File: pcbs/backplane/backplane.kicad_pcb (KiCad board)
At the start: 2 copper layers, 80 x 50 mm, 11 parts, among them P1 CONN_02X04, P2 CONN_02X04, P3 USB_B, P4 CONN_02X09, P5 CONN_02X09, U1 FT232RL

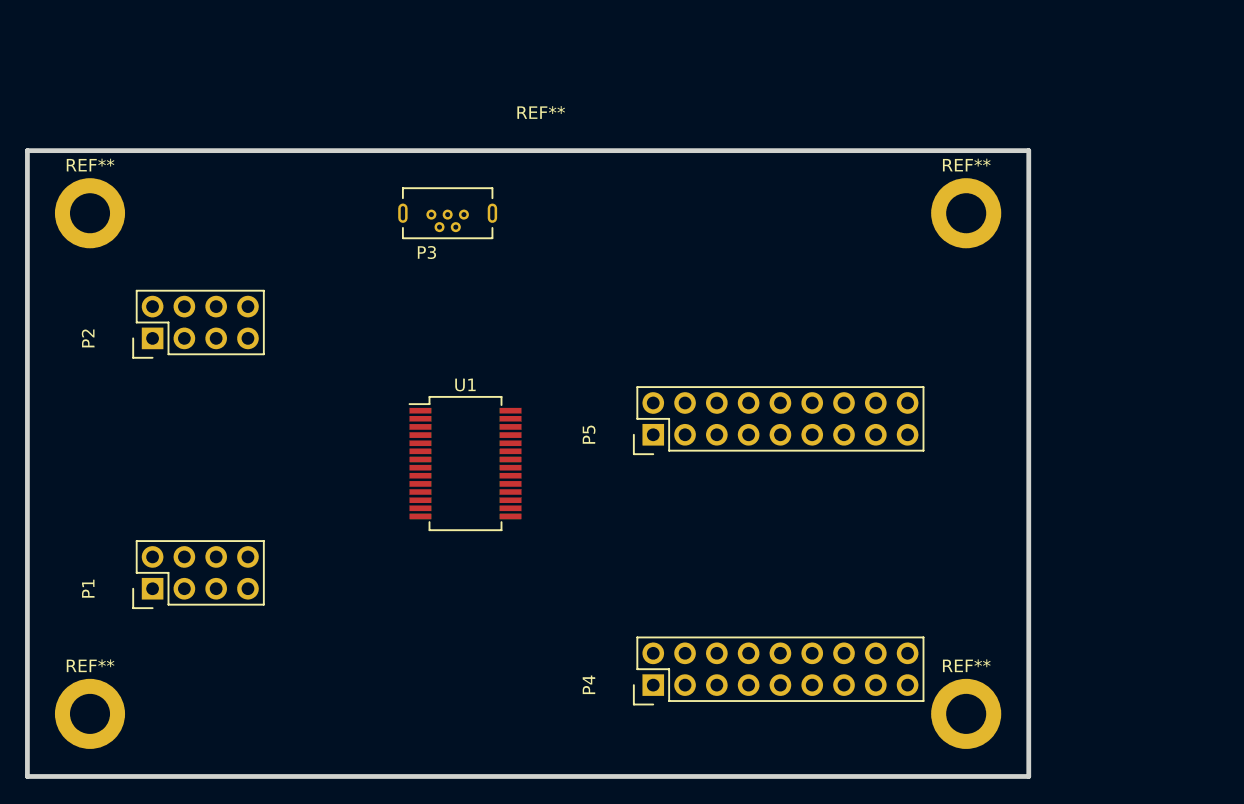
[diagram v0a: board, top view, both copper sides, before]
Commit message: Mechanical specs updated.
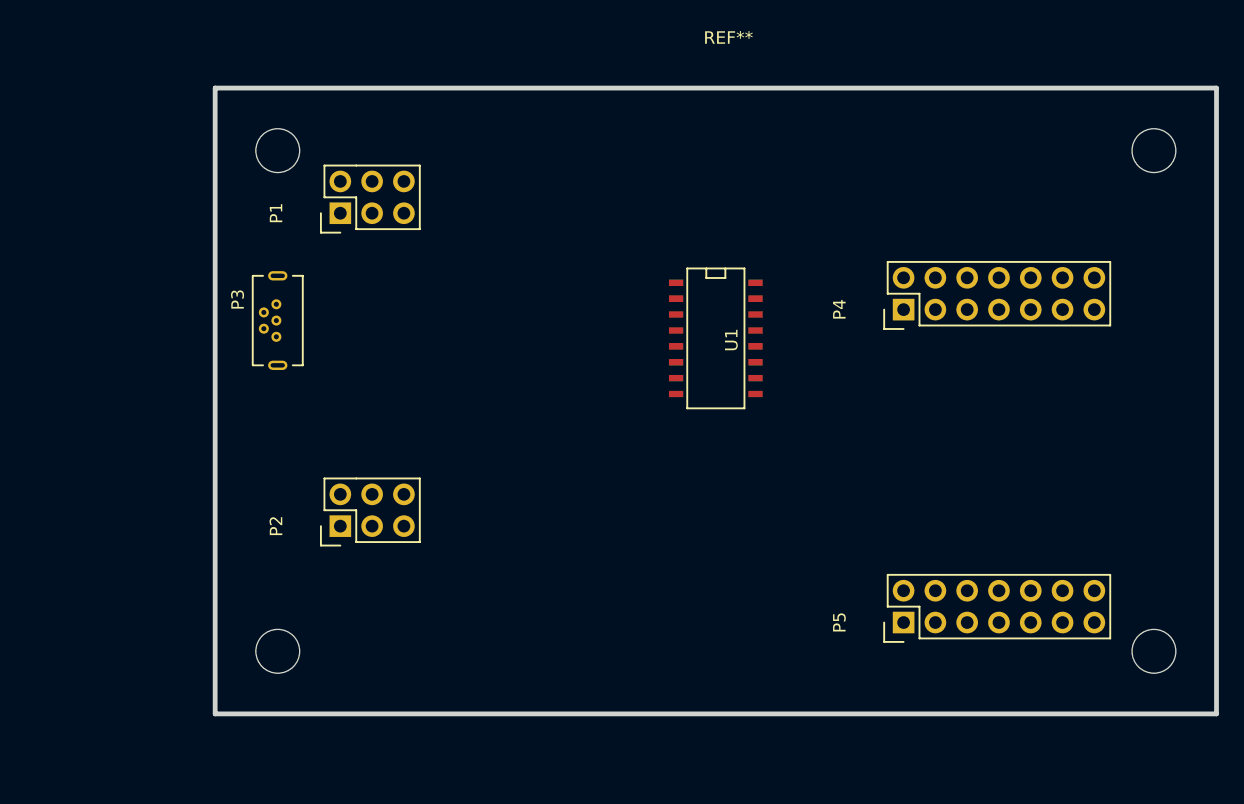
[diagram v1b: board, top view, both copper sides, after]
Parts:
- removed the REF** at (95.0, 125.0)
- removed the REF** at (100.0, 80.0)
- removed the REF** at (100.0, 120.0)
- removed the REF** at (170.0, 120.0)
- removed the REF** at (170.0, 80.0)
- added REF**: EuroBoard_viertel_Type-I_80mmX50mm_holes, EuroBoard_Outline:EuroBoard_viertel_Type-I_80mmX50mm_holes, F.Cu at (110.0, 120.0)
- P1, P2: value CONN_02X04 -> CONN_02X03; footprint Pin_Headers:Pin_Header_Straight_2x04 -> Pin_Headers:Pin_Header_Straight_2x03
- P4, P5: value CONN_02X09 -> CONN_02X07; footprint Pin_Headers:Pin_Header_Straight_2x09 -> Pin_Headers:Pin_Header_Straight_2x07
- U1: value FT232RL -> CH340G; footprint Housings_SSOP:SSOP-28_5.3x10.2mm_Pitch0.65mm -> SMD_Packages:SO-16-N
- moved P4 36.1 mm to (165.0, 87.7)
- moved P1 33.5 mm to (120.0, 80.0)
- moved P5 25.0 mm to (165.0, 112.7)
- moved U1 22.4 mm to (150.0, 90.0), turned to 270 degrees
- moved P2 21.2 mm to (120.0, 105.0)
- moved P3 11.2 mm to (115.0, 85.0), turned to 270 degrees
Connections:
- net PWM1 renamed GPIO0
- net SPI_CS renamed UART_RX
- net VCC renamed 5V
- P1 pad 4: GND -> ADC3
- P1 pad 6: DAC1 -> ADC4
- P2 pad 4: GND -> ADC3
- P2 pad 6: DAC1 -> ADC4
- P4 pad 10: GPIO1 -> GPIO4
- P4 pad 12: GPIO2 -> nRST
- P4 pad 13: I2C_SCL -> DAC1
- P4 pad 14: GPIO3 -> DAC2
- P4 pad 4: PWM2 -> GPIO1
- P4 pad 5: SPI_CLK -> I2C_SCL
- P4 pad 6: DAC1 -> GPIO2
- P4 pad 7: SPI_MISO -> I2C_SDA
- P4 pad 8: DAC2 -> GPIO3
- P4 pad 9: SPI_MOSI -> UART_TX
- P5 pad 10: GPIO1 -> GPIO4
- P5 pad 12: GPIO2 -> nRST
- P5 pad 13: I2C_SCL -> DAC1
- P5 pad 14: GPIO3 -> DAC2
- P5 pad 4: PWM2 -> GPIO1
- P5 pad 5: SPI_CLK -> I2C_SCL
- P5 pad 6: DAC1 -> GPIO2
- P5 pad 7: SPI_MISO -> I2C_SDA
- P5 pad 8: DAC2 -> GPIO3
- P5 pad 9: SPI_MOSI -> UART_TX
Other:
- board text added: "The boards, which are plugged in should have the right angeled mates at the edge."
- board text added: "This is the distance one has between the two boards minus the board thickness and the highest component."
